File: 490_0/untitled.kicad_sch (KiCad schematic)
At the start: 37 parts, among them J2 BM04B-PASS-1-TFT, J3 BM04B-PASS-1-TFT, U2 TPS2553DBVR, U3 TPS2553DBVR, U4 USB2512B-I/M2, Y1 24 MHz

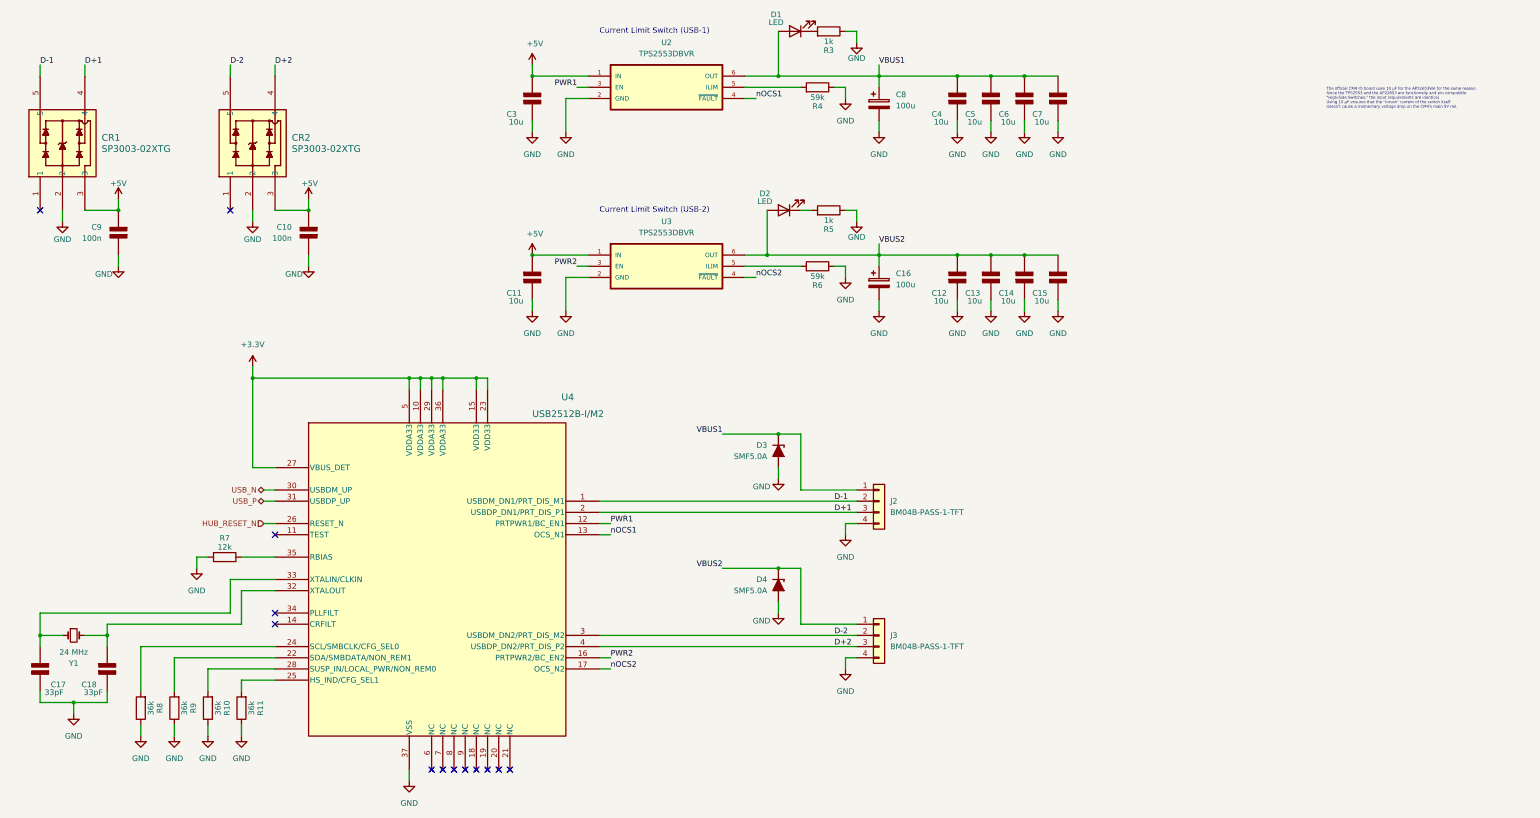
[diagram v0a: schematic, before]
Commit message: USB hub fix
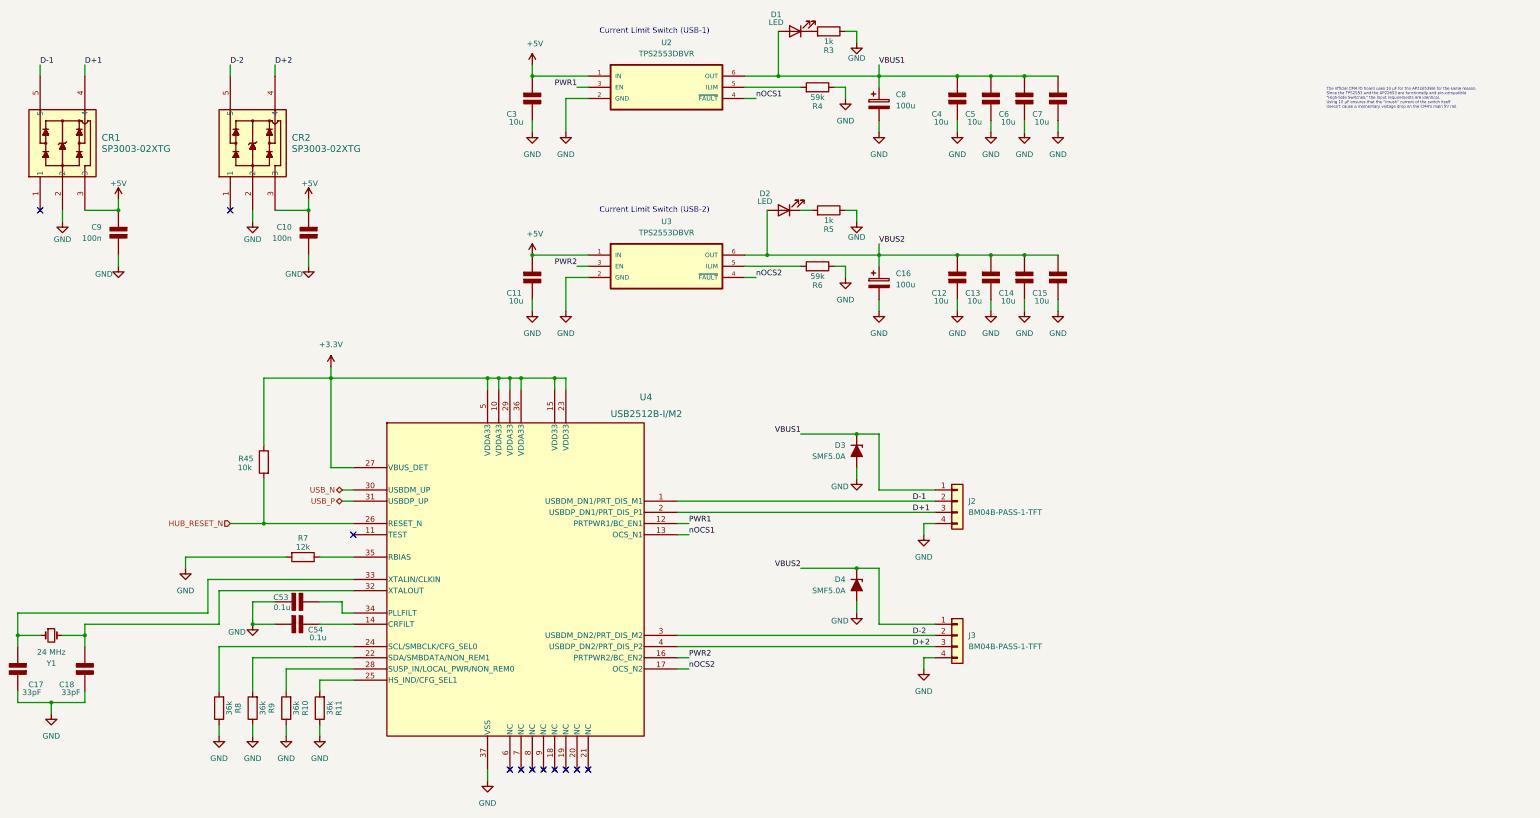
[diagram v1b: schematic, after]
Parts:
- added C53, C54: 0.1u, symbol PCM_Elektuur:C
- added R45: 10k, symbol Device:R
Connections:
- net +3.3V: now also R45.1
- net GND: now also C53.1 (+), C54.1 (+)
- net HUB_RESET_N: now also R45.2
- net at U4.14 (CRFILT): now also C54.2 (-)
- net at U4.34 (PLLFILT): now also C53.2 (-)
- no-connect marks 13 -> 11
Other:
- moved on the sheet: C17, C18, D3, D4, J2, J3, R10, R11, R7, R8, R9, U4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
